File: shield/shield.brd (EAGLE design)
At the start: 68.6 x 53.3 mm, 26 parts, among them IC1 MCP2515-E/SO, IC2 MCP2562, IC3 LM2595NDH, IC4 PESD1CAN

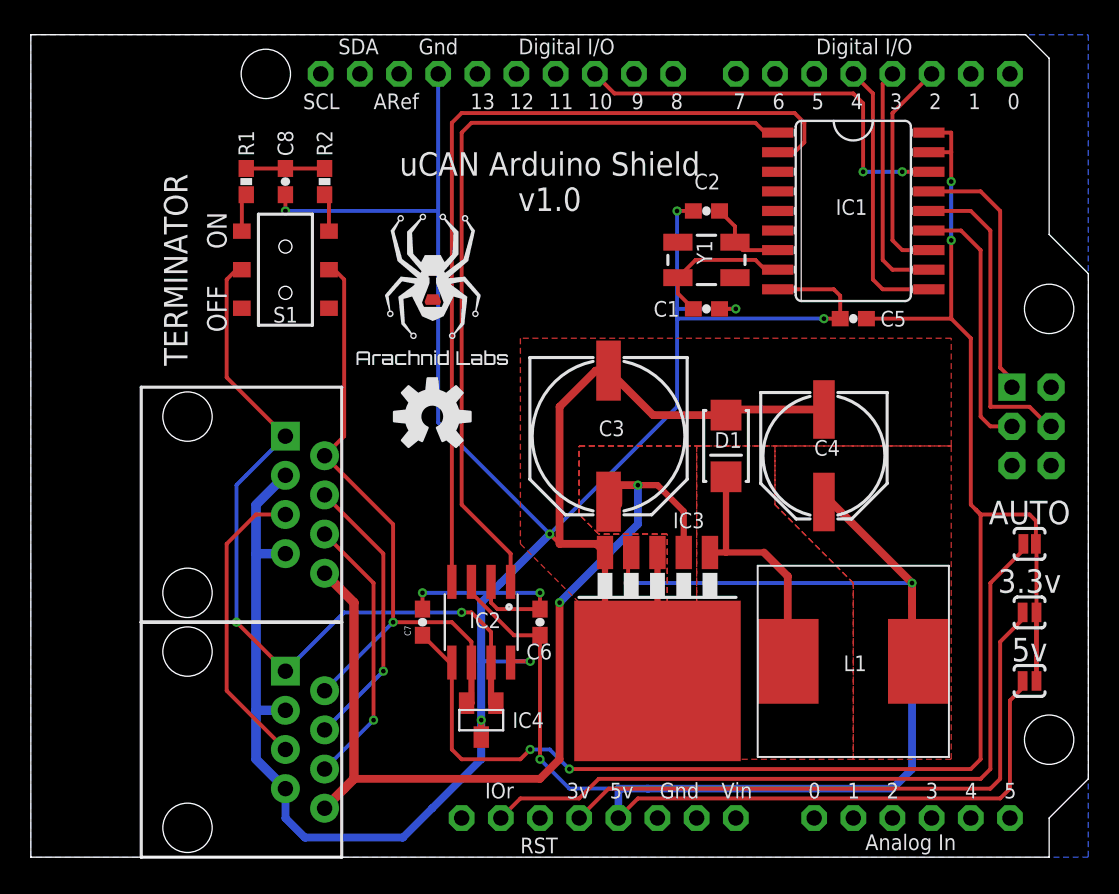
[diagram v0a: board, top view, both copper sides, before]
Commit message: Minor changes to shield, rpi board, and cape
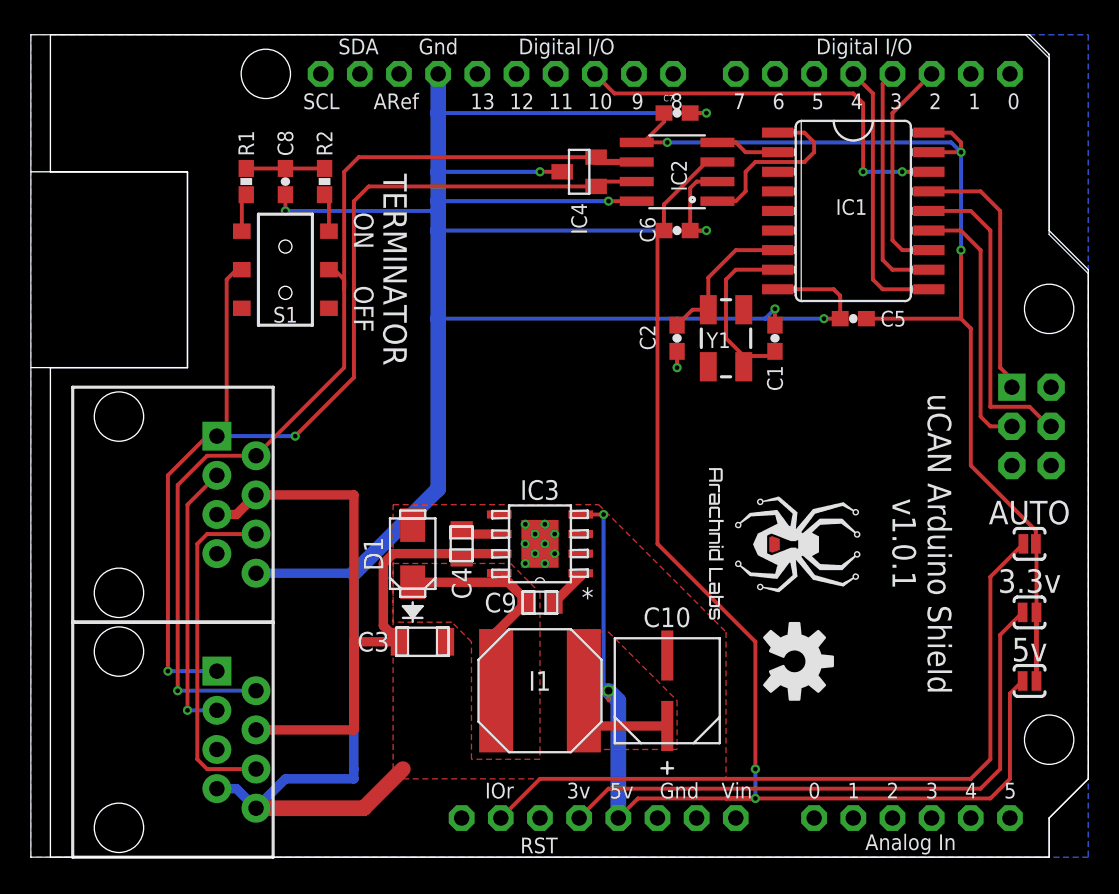
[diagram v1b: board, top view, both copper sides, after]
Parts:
- removed L1: MSS1260, nickparts:MSS1260
- added C10: 56u, nickparts:SM_RADIAL_6.3AMM
- added C9: 10n, nickparts:0805
- added I1: SRN8040-330M, nickparts:SRN8040
- C3: value (none) -> 4.7u; device SparkFun-Capacitors:PANASONIC_G -> nickparts:1206
- C4: value (none) -> 1u; device SparkFun-Capacitors:PANASONIC_E -> nickparts:0805
- D1: value (none) -> B240A-13-F; device SparkFun-DiscreteSemi:SMA-DIODE_ALT -> nickparts:SMA
- IC3: value LM2595NDH -> LM22675MR-5.0/NOPB; device nickparts:TO263-5 -> nickparts:MRA08B
- U$1: value ARDUINO_R3_ICSP -> ARDUINO_R3_ICSPNODIM; device adafruit:ARDUINOR3_ICSP -> nickparts:ARDUINOR3_ICSP_NODIM
- moved C7 36.9 mm to (41.9, 48.3), turned to 0 degrees
- moved IC4 36.1 mm to (35.6, 44.5), turned to 90 degrees
- moved IC2 31.9 mm to (41.9, 44.5), turned to 90 degrees
- moved U$5 28.4 mm to (49.5, 12.7), turned to 270 degrees
- moved U$4 28.2 mm to (48.9, 20.3), turned to 270 degrees
- moved C6 26.9 mm to (41.9, 40.6), turned to 0 degrees
- moved C4 24.2 mm to (27.9, 20.3), turned to 90 degrees
- moved D1 21.5 mm to (24.8, 19.7), turned to 90 degrees
- moved C3 18.0 mm to (25.4, 14.0), turned to 0 degrees
- moved IC3 9.92 mm to (33.0, 20.3)
- moved C2 8.47 mm to (41.9, 33.7), turned to 270 degrees
- moved Y1 5.24 mm to (45.1, 33.7), turned to 270 degrees
- moved C1 4.84 mm to (48.3, 33.7), turned to 90 degrees
- moved U$2 4.45 mm to (5.71, 22.9)
- moved U$3 4.45 mm to (5.71, 7.62)
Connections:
- net N$1 renamed RXCAN
- removed net N$11: U$2.5, U$3.5
- removed net N$6: D1.C, IC3.1, L1.P$1
- new net N$9: U$2.3, U$3.3
- new net SWOUT: C9.2, D1.1, I1.2, IC3.8
- net +5V: now also C10.1, I1.1; no longer C4.+, L1.P$2
- net GND: now also C10.2, C3.2, C4.2, D1.2, IC3.EPAD, U$2.8, U$3.8; no longer C3.-, C4.-, D1.A, IC3.3, IC3.5, U$2.3, U$3.3
- net N$10: now also C9.1, IC3.1; no longer U$2.4, U$3.4
- net VCC: now also C3.1, C4.1, IC3.7, U$2.4, U$2.5, U$3.4, U$3.5; no longer C3.+, IC3.2, U$2.8, U$3.8
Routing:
- net RXCAN: track 56.8 -> 4.53 mm
- net TXCAN: track 51.5 -> 11.6 mm
- net V+: track 112.8 -> 75.7 mm, vias 4 -> 3
- net GND: track 224.6 -> 189.1 mm, vias 9 -> 18
- net CANL: track 42.0 -> 66.6 mm
- net CANH: track 51.2 -> 72.5 mm
- net N$11: track 19.5 -> 0.00 mm
- net N$9: track 0.00 -> 17.9 mm, vias 0 -> 1
- net N$6: track 16.1 -> 0.00 mm
- net SWOUT: track 0.00 -> 15.9 mm
- net N$10: track 18.4 -> 2.62 mm, vias 1 -> 0
- net +5V: track 122.2 -> 111.3 mm, vias 3 -> 4
- net VCC: track 62.2 -> 53.4 mm, vias 2 -> 0
- net N$5: track 5.43 -> 9.76 mm
- net N$8: track 17.9 -> 22.1 mm, vias 1 -> 0
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- added copper zone on layer 1, net SWOUT
- removed copper zone on layer 1, net N$6
- removed copper zone on layer 1, net VCC
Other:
- outline, holes or cut-outs redrawn
- board text added: "uCAN Arduino Shield v1.0.1"
- board text removed: "uCAN Arduino Shield v1.0"
